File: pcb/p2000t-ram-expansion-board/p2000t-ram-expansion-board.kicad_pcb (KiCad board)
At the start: 2 copper layers, 11 parts, among them J1 EXTENSION BOARD, U1 74HC04, U10 74HC32, U2 CY62256-70PC, U3 74HC32, U4 CY62256-70PC, U5 74HC688, U6 74HC04, U7 74HC08, U8 74HC173, U9 74HC08

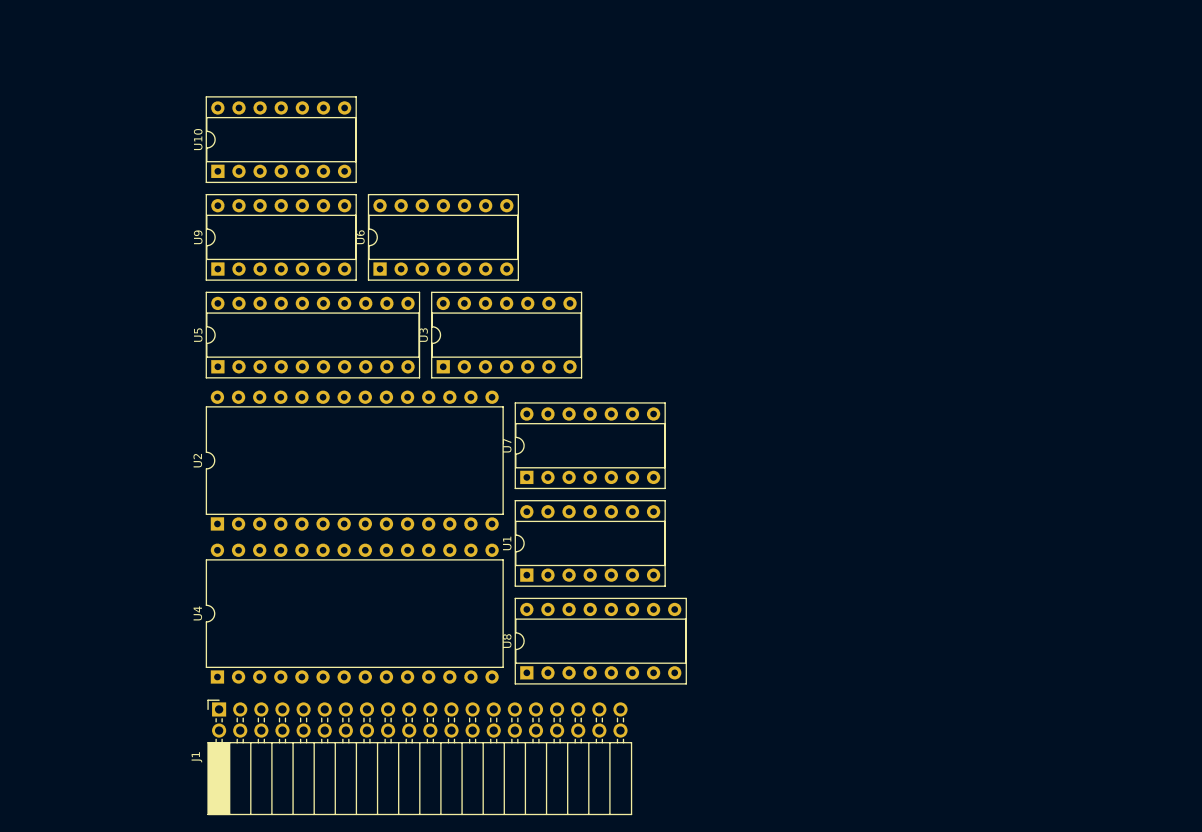
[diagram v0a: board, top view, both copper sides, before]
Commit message: Revising design
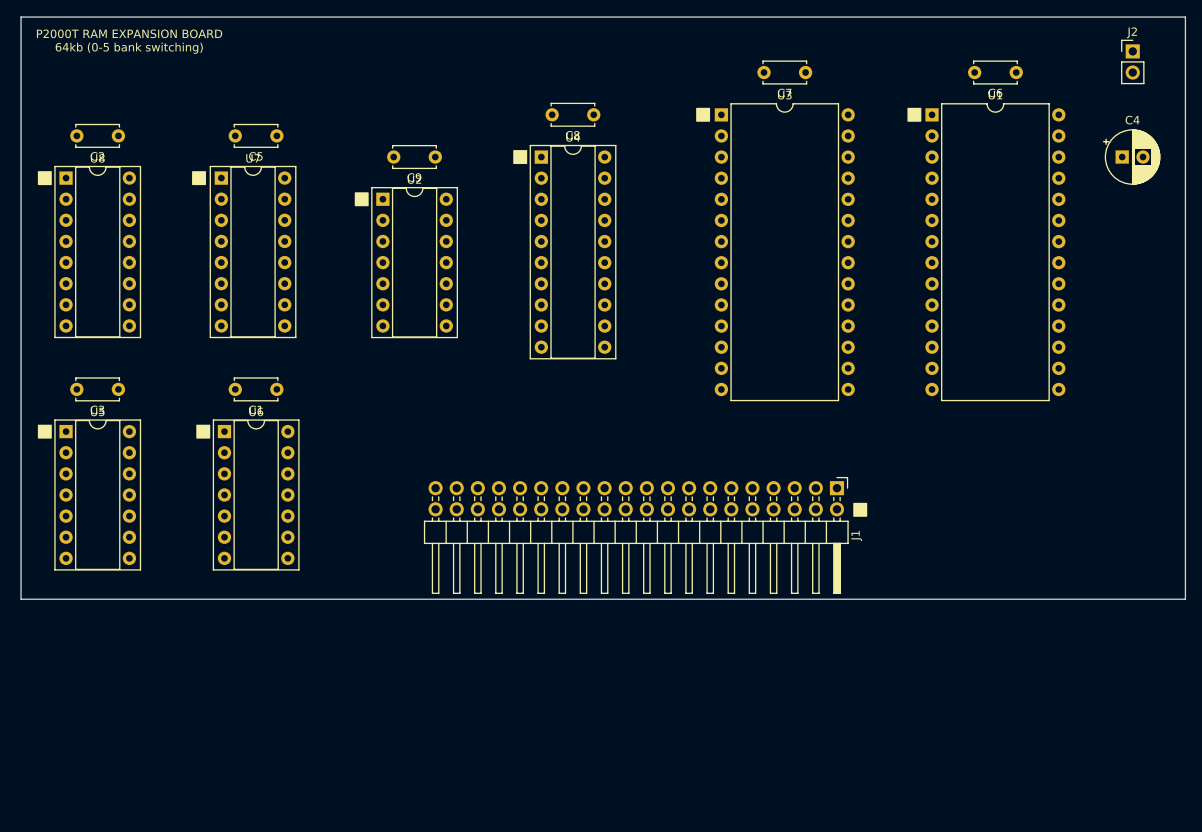
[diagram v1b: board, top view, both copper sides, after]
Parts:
- removed the U1 at (80.8, 87.1)
- removed U10: 74HC32, Package_DIP:DIP-14_W7.62mm_Socket
- removed the U3 at (70.8, 62.1)
- removed the U7 at (80.8, 75.4)
- removed U9: 74HC08, Package_DIP:DIP-14_W7.62mm_Socket
- added C1: 0.1uF, Capacitor_THT:C_Disc_D5.0mm_W2.5mm_P5.00mm, F.Cu at (50.8, 64.8)
- added C2: 0.1uF, Capacitor_THT:C_Disc_D5.0mm_W2.5mm_P5.00mm, F.Cu at (31.7, 34.3)
- added C3: 0.1uF, Capacitor_THT:C_Disc_D5.0mm_W2.5mm_P5.00mm, F.Cu at (31.7, 64.8)
- added C4: 220uF, Capacitor_THT:CP_Radial_D6.3mm_P2.50mm, F.Cu at (152.4, 36.8)
- added C5: 0.1uF, Capacitor_THT:C_Disc_D5.0mm_W2.5mm_P5.00mm, F.Cu at (50.8, 34.3)
- added C6: 0.1uF, Capacitor_THT:C_Disc_D5.0mm_W2.5mm_P5.00mm, F.Cu at (139.7, 26.7)
- added C7: 0.1uF, Capacitor_THT:C_Disc_D5.0mm_W2.5mm_P5.00mm, F.Cu at (114.3, 26.7)
- added C8: 0.1uF, Capacitor_THT:C_Disc_D5.0mm_W2.5mm_P5.00mm, F.Cu at (88.9, 31.8)
- added C9: 0.1uF, Capacitor_THT:C_Disc_D5.0mm_W2.5mm_P5.00mm, F.Cu at (69.8, 36.8)
- added J2: POWER, Connector_PinHeader_2.54mm:PinHeader_1x02_P2.54mm_Vertical, F.Cu at (153.7, 24.1)
- added U2: 74HC00, Package_DIP:DIP-14_W7.62mm_Socket, F.Cu at (63.5, 41.9)
- added U5: 74HC00, Package_DIP:DIP-14_W7.62mm_Socket, F.Cu at (25.4, 69.8)
- added U8: 74LHC157, Package_DIP:DIP-16_W7.62mm_Socket, F.Cu at (25.4, 39.4)
- J1: value EXTENSION BOARD -> EXPANSION BOARD; footprint Connector_PinSocket_2.54mm:PinSocket_2x20_P2.54mm_Horizontal -> Connector_PinHeader_2.54mm:PinHeader_2x20_P2.54mm_Horizontal
- U6: value 74HC04 -> 74HC32
- moved U1 99.0 mm to (129.5, 31.8), turned to 0 degrees
- moved U3 90.8 mm to (104.2, 31.8), turned to 0 degrees
- moved J1 78.9 mm to (118.1, 76.6), turned to -90 degrees
- moved U7 69.9 mm to (44.1, 39.4), turned to 0 degrees
- moved U4 46.4 mm to (82.6, 36.8), turned to 0 degrees
- moved U6 27.1 mm to (44.5, 69.8), turned to 0 degrees
- renumbered U2 to U1, U4 to U3, U5 to U4, U8 to U7
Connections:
- J1 pad 10: D7 -> D6
- J1 pad 11: A0 -> A1
- J1 pad 12: A1 -> A0
- J1 pad 13: A2 -> A3
- J1 pad 14: A3 -> A2
- J1 pad 15: A4 -> A5
- J1 pad 16: A5 -> A4
- J1 pad 17: A6 -> A7
- J1 pad 18: A7 -> A6
- J1 pad 19: A8 -> A9
- J1 pad 2: unconnected-(J1-Pad2) -> GND
- J1 pad 20: A9 -> A8
- J1 pad 21: A10 -> A11
- J1 pad 22: A11 -> A10
- J1 pad 23: A12 -> A13
- J1 pad 24: A13 -> A12
- J1 pad 25: A14 -> RAMS2
- J1 pad 26: RAMS2 -> A14
- J1 pad 27: ~{MRQ} -> ~{RD}
- J1 pad 28: ~{RD} -> ~{MRQ}
- J1 pad 29: unconnected-(J1-Pad29) -> ~{WR}
- J1 pad 3: D0 -> D1
- J1 pad 30: ~{WR} -> unconnected-(J1-Pad30)
- J1 pad 31: ~{IORQ} -> unconnected-(J1-Pad31)
- J1 pad 32: unconnected-(J1-Pad32) -> ~{IORQ}
- J1 pad 33: unconnected-(J1-Pad33) -> ~{RES}
- J1 pad 34: ~{RES} -> unconnected-(J1-Pad34)
- J1 pad 4: D1 -> D0
- J1 pad 5: D2 -> D3
- J1 pad 6: D3 -> D2
- J1 pad 7: D4 -> D5
- J1 pad 8: D5 -> D4
- J1 pad 9: D6 -> D7
- U1 pad 1: A14P -> A14_1
- U1 pad 20: Net-(U2-Pad20) -> ~{CS1}
- U1 pad 26: A13P -> A13_1
- U3 pad 1: A14P -> A14_2
- U3 pad 20: Net-(U3-Pad8) -> ~{CS2}
- U3 pad 26: A13P -> A13_2
- U6 pad 1: (no net) -> Net-(U5-Pad3)
- U6 pad 10: (no net) -> S2
- U6 pad 11: (no net) -> ~{CS1}
- U6 pad 12: (no net) -> Net-(U5-Pad11)
- U6 pad 13: (no net) -> ~{REN}
- U6 pad 2: (no net) -> ~{REN}
- U6 pad 3: (no net) -> ~{CS2}
- U6 pad 4: (no net) -> Net-(U5-Pad6)
- U6 pad 5: (no net) -> Net-(U5-Pad8)
- U6 pad 6: (no net) -> Net-(U5-Pad12)
- U6 pad 8: (no net) -> Net-(U6-Pad8)
- U6 pad 9: (no net) -> S1
- U7 pad 11: GND -> D3
- U7 pad 15: Net-(U1-Pad12) -> RES
- U7 pad 7: Net-(U8-Pad7) -> WR
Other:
- board outline added: 140 x 70 mm
- board text added: "P2000T RAM EXPANSION BOARD 64kb (0-5 bank switching)"
